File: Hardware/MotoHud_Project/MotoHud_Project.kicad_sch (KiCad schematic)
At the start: 9 parts, among them J1 I2C, J2 BAT CHARGER, J3 Conn_01x02_Pin, J4 BTN

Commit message: updated rxver and txver hardware
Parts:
- R1, R2: footprint Resistor_THT:R_Axial_DIN0207_L6.3mm_D2.5mm_P7.62mm_Horizontal -> Resistor_SMD:R_0603_1608Metric_Pad0.98x0.95mm_HandSolder
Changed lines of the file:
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@@
 			)
 		)
-		(property "Footprint" "Resistor_THT:R_Axial_DIN0207_L6.3mm_D2.5mm_P7.62mm_Horizontal"
+		(property "Footprint" "Resistor_SMD:R_0603_1608Metric_Pad0.98x0.95mm_HandSolder"
 			(at 153.67 58.42 0)
 			(effects
@@
 			)
 		)
-		(property "Footprint" "Resistor_THT:R_Axial_DIN0207_L6.3mm_D2.5mm_P7.62mm_Horizontal"
+		(property "Footprint" "Resistor_SMD:R_0603_1608Metric_Pad0.98x0.95mm_HandSolder"
 			(at 153.67 52.07 0)
 			(effects

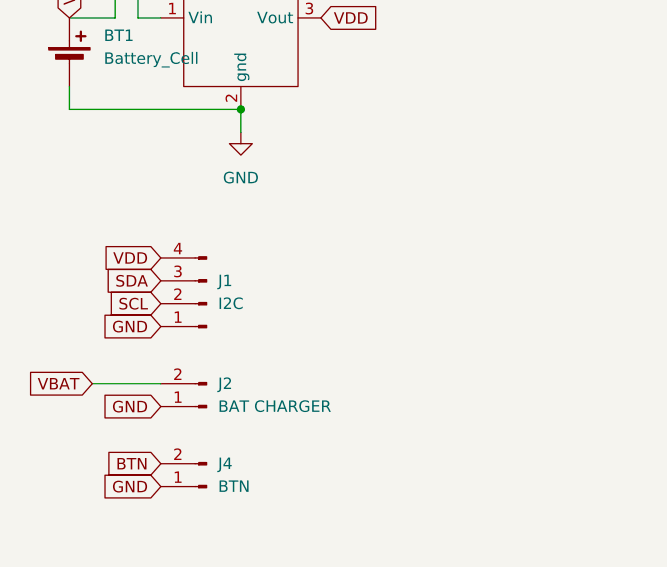
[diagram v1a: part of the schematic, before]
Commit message: updated hardware
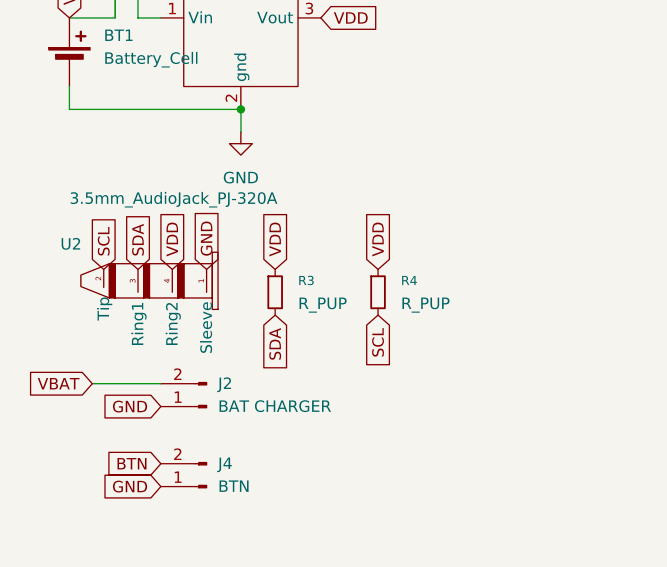
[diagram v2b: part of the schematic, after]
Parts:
- removed J1: I2C, Connector_PinHeader_2.54mm:PinHeader_1x04_P2.54mm_Vertical, symbol Connector:Conn_01x04_Pin
- added R3, R4: R_PUP, Resistor_THT:R_Axial_DIN0207_L6.3mm_D2.5mm_P10.16mm_Horizontal, symbol Device:R_Small
- added U2: 3.5mm_AudioJack_PJ-320A, CUSTOM_MODULES:3.5mm_AudioJack_PJ-320A_NoGuide, symbol CUSTOM_MODULE:3.5mm_AudioJack_PJ-320A
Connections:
- net GND: now also U2.1 (Sleeve)
- net SCL: now also R4.2, U2.2 (Tip)
- net SDA: now also R3.2, U2.3 (Ring1)
- net VDD: now also R3.1, R4.1, U2.4 (Ring2)
